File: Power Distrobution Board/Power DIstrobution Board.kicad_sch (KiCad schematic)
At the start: 2 parts, among them J2 Conn_01x10_Pin, J4 Conn_01x04_Pin

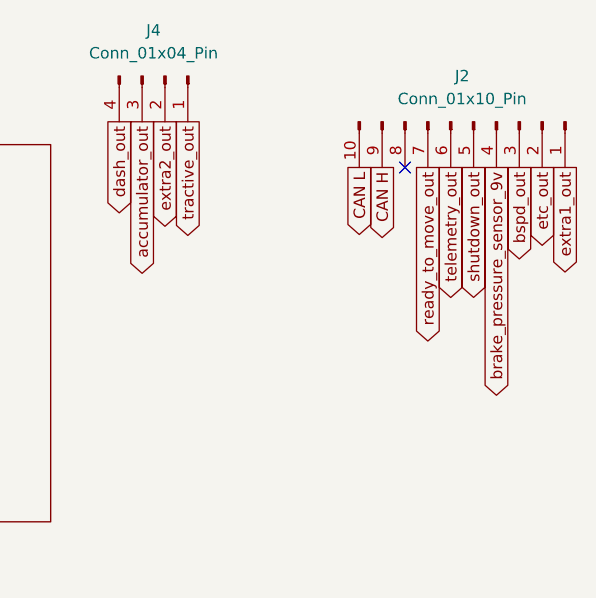
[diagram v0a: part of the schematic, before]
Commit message: version 1.1
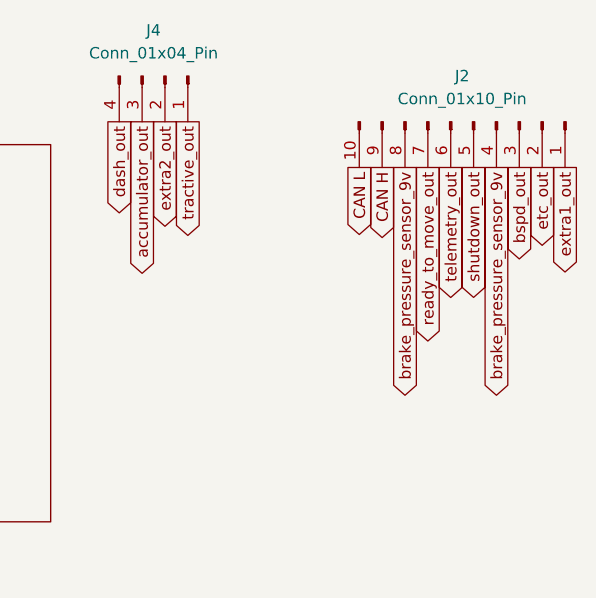
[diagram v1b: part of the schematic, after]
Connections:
- net brake_pressure_sensor_9v: now also J2.8 (Pin_8)
- no-connect marks 1 -> 0
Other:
- company: (none) -> Formula Slug
- title: (none) -> PD BOARD
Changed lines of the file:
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@@
 	(generator_version "8.0")
 	(paper "A4")
-	(no_connect
-		(at 262.89 71.12)
+	(title_block
+		(title "PD BOARD")
+		(date "2024-11-11")
+		(rev "1.1")
+		(company "Formula Slug")
 	)
 	(global_label "CAN H"
@@
 		)
 	)
+	(global_label "brake_pressure_sensor_9v"
+		(shape output)
+		(at 273.05 71.12 270)
+		(fields_autoplaced yes)
+		(effects
+			(font
+				(size 1.27 1.27)
+			)
+			(justify right)
+		)
+		(property "Intersheetrefs" "${INTERSHEET_REFS}"
+			(at 273.05 98.7188 90)
+			(effects
+				(font
+					(size 1.27 1.27)
+				)
+				(justify right)
+				(hide yes)
+			)
+		)
+	)
+	(global_label "brake_pressure_sensor_9v"
+		(shape output)
+		(at 262.89 71.12 270)
+		(fields_autoplaced yes)
+		(effects
+			(font
+				(size 1.27 1.27)
+			)
+			(justify right)
+		)
+		(property "Intersheetrefs" "${INTERSHEET_REFS}"
+			(at 262.89 98.7188 90)
+			(effects
+				(font
+					(size 1.27 1.27)
+				)
+				(justify right)
+				(hide yes)
+			)
+		)
+	)
 	(global_label "dash_out"
 		(shape output)
@@
 			(effects
 				(font
-					(size 1.27 1.27)
-				)
-				(justify right)
-				(hide yes)
-			)
-		)
-	)
-	(global_label "brake_pressure_sensor_9v"
-		(shape output)
-		(at 273.05 71.12 270)
-		(fields_autoplaced yes)
-		(effects
-			(font
-				(size 1.27 1.27)
-			)
-			(justify right)
-		)
-		(property "Intersheetrefs" "${INTERSHEET_REFS}"
-			(at 273.05 98.7188 90)
-			(effects
-				(font

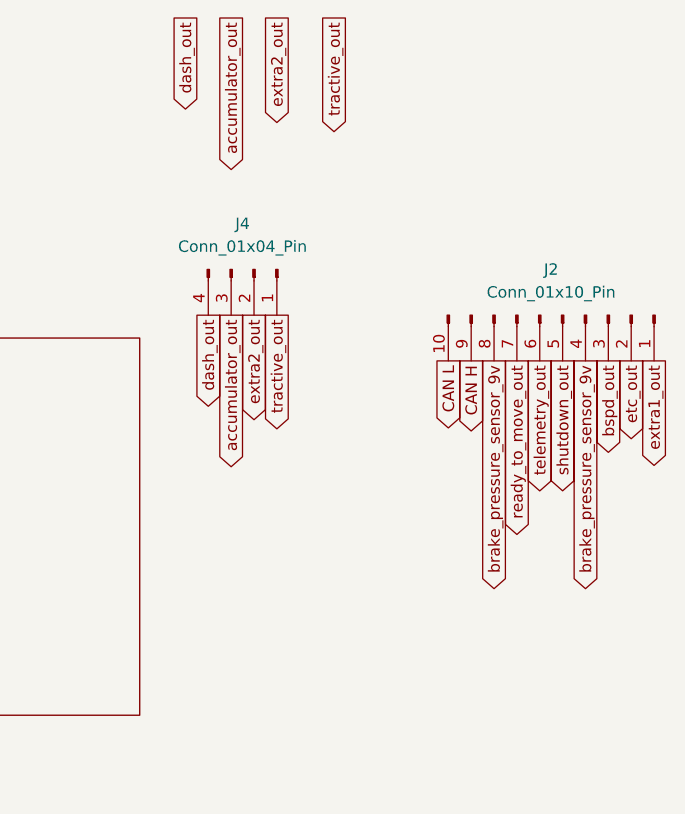
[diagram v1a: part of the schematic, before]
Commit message: even newer changes
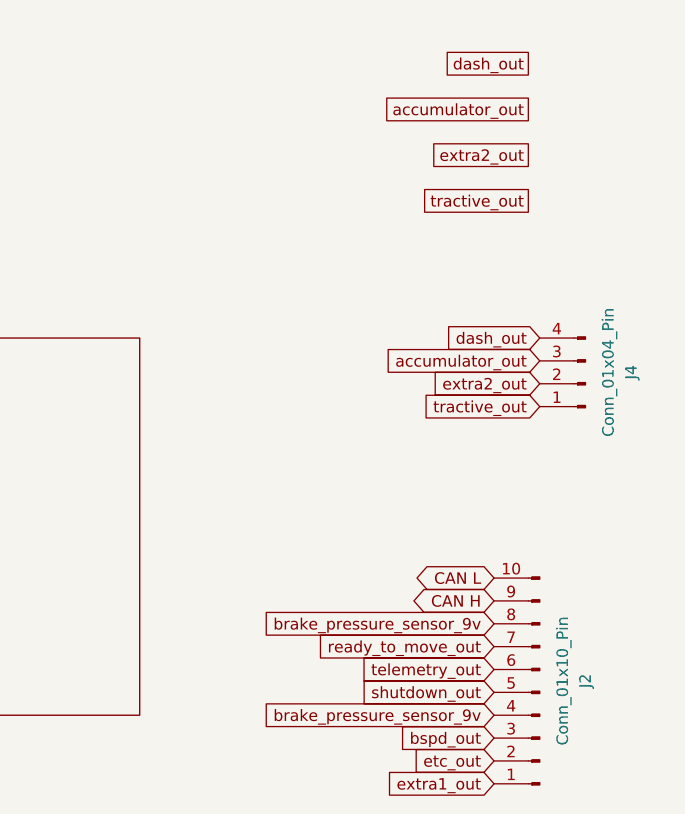
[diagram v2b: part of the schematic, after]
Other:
- moved on the sheet: J2, J4

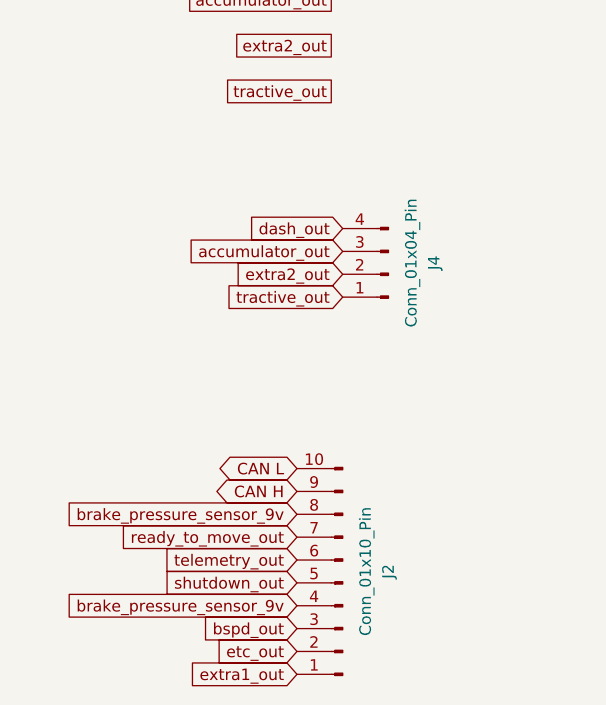
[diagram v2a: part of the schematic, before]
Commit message: commit 1 of v2
pd board v2 work first commit
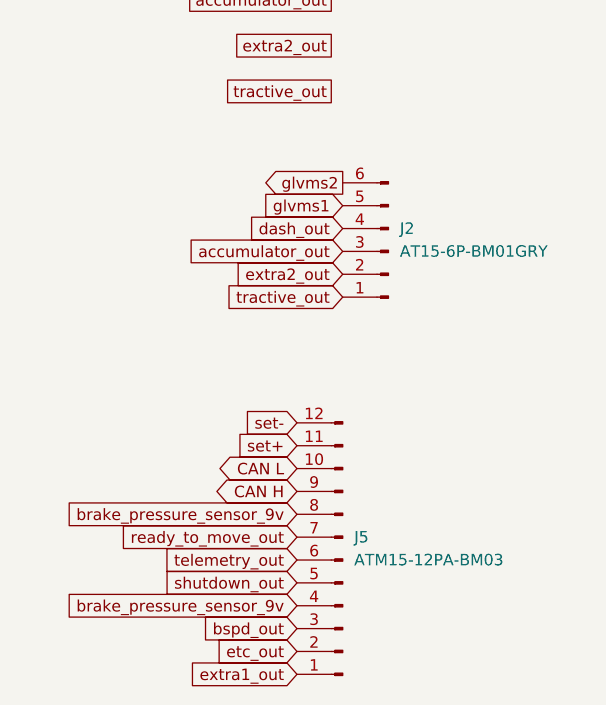
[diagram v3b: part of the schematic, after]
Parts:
- removed J2: Conn_01x10_Pin, Connector_Molex:Molex_Nano-Fit_105314-xx10_2x05_P2.50mm_Horizontal, symbol Connector:Conn_01x10_Pin
- removed J4: Conn_01x04_Pin, Connector_Molex:Molex_Mega-Fit_76825-0004_2x02_P5.70mm_Horizontal, symbol Connector:Conn_01x04_Pin
- added J2: AT15-6P-BM01GRY, FS_3_Global_Footprint_Library:CONN6_DT15-6P_TEC, symbol Connector:Conn_01x06_Pin
- added J5: ATM15-12PA-BM03, FS_3_Global_Footprint_Library:TE_DTM15-12PA, symbol Connector:Conn_01x12_Pin
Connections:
- net CAN H: now also J5.9 (Pin_9)
- net CAN L: now also J5.10 (Pin_10)
- net accumulator_out: now also J2.3 (Pin_3)
- net brake_pressure_sensor_9v: now also J5.4 (Pin_4), J5.8 (Pin_8)
- net bspd_out: now also J5.3 (Pin_3)
- net dash_out: now also J2.4 (Pin_4)
- net etc_out: now also J5.2 (Pin_2)
- net extra1_out: now also J5.1 (Pin_1)
- net extra2_out: now also J2.2 (Pin_2)
- net ready_to_move_out: now also J5.7 (Pin_7)
- net shutdown_out: now also J5.5 (Pin_5)
- net telemetry_out: now also J5.6 (Pin_6)
- net tractive_out: now also J2.1 (Pin_1)
- new net glvms1: J2.5 (Pin_5)
- new net glvms2: J2.6 (Pin_6)
- new net set+: J5.11 (Pin_11)
- new net set-: J5.12 (Pin_12)
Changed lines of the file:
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@@
+		)
+	)
+	(global_label "extra1_out"
+		(shape input)
+		(at 262.89 118.11 180)
+		(fields_autoplaced yes)
+		(effects
+			(font
+				(size 1.27 1.27)
+			)
+			(justify right)
+		)
+		(property "Intersheetrefs" "${INTERSHEET_REFS}"
+			(at 249.9264 118.11 0)
+			(effects
+				(font
+					(size 1.27 1.27)
+				)
+				(justify right)
+				(hide yes)
+			)
 		)
 	)
@@
 		)
 	)
-	(global_label "extra1_out"
-		(shape input)
-		(at 262.89 118.11 180)
-		(fields_autoplaced yes)
-		(effects
-			(font
-				(size 1.27 1.27)
-			)
-			(justify right)
-		)
-		(property "Intersheetrefs" "${INTERSHEET_REFS}"
-			(at 249.9264 118.11 0)
-			(effects
-				(font
-					(size 1.27 1.27)
-				)
-				(justify right)
-				(hide yes)
-			)
-		)
-	)
 	(global_label "etc_out"
 		(shape input)
@@
 		(property "Intersheetrefs" "${INTERSHEET_REFS}"
 			(at 253.0106 115.57 0)
+			(effects
+				(font
+					(size 1.27 1.27)
+				)
+				(justify right)
+				(hide yes)
+			)
+		)
+	)
+	(global_label "glvms1"
+		(shape input)
+		(at 267.97 66.04 180)
+		(fields_autoplaced yes)
+		(effects
+			(font
+				(size 1.27 1.27)
+			)
+			(justify right)
+		)
+		(property "Intersheetrefs" "${INTERSHEET_REFS}"
+			(at 258.2721 66.04 0)
 			(effects
 				(font
@@
 		)
 	)
+	(global_label "set+"
+		(shape input)
+		(at 262.89 92.71 180)
+		(fields_autoplaced yes)
+		(effects
+			(font
+				(size 1.27 1.27)
+			)
+			(justify right)
+		)
+		(property "Intersheetrefs" "${INTERSHEET_REFS}"
+			(at 255.49 92.71 0)
+			(effects
+				(font
+					(size 1.27 1.27)
+				)
+				(justify right)
+				(hide yes)
+			)
+		)
+	)
 	(global_label "ready_to_move_out"
 		(shape input)
@@
 		)
 	)
+	(global_label "glvms2"
+		(shape output)
+		(at 267.97 63.5 180)
+		(fields_autoplaced yes)
+		(effects
+			(font
+				(size 1.27 1.27)
+			)
+			(justify right)
+		)
+		(property "Intersheetrefs" "${INTERSHEET_REFS}"
+			(at 258.2721 63.5 0)
+			(effects
+				(font
+					(size 1.27 1.27)
+				)
+				(justify right)
+				(hide yes)
+			)
+		)
+	)
 	(global_label "shutdown_out"
 		(shape input)
@@
 		(property "Intersheetrefs" "${INTERSHEET_REFS}"
 			(at 253.8573 76.2 0)
+			(effects
+				(font
+					(size 1.27 1.27)
+				)
+				(justify right)
+				(hide yes)
+			)
+		)
+	)
+	(global_label "set-"
+		(shape input)
+		(at 262.89 90.17 180)
+		(fields_autoplaced yes)
+		(effects
+			(font
+				(size 1.27 1.27)
+			)
+			(justify right)
+		)
+		(property "Intersheetrefs" "${INTERSHEET_REFS}"
+			(at 255.49 90.17 0)
 			(effects
 				(font
@@
 	)
 	(symbol
-		(lib_id "Connector:Conn_01x10_Pin")
-		(at 267.97 107.95 180)
+		(lib_id "Connector:Conn_01x12_Pin")
+		(at 267.97 105.41 180)
 		(unit 1)
 		(exclude_from_sim no)
@@
 		(dnp no)
 		(fields_autoplaced yes)
+		(property "Reference" "J5"
+			(at 269.24 102.8699 0)
+			(effects
+				(font
+					(size 1.27 1.27)
+				)
+				(justify right)
+			)
+		)
+		(property "Value" "ATM15-12PA-BM03"
+			(at 269.24 105.4099 0)
+			(effects
+				(font
+					(size 1.27 1.27)
+				)
+				(justify right)
+			)
+		)
+		(property "Footprint" "FS_3_Global_Footprint_Library:TE_DTM15-12PA"
+			(at 267.97 105.41 0)
+			(effects
+				(font
+					(size 1.27 1.27)
+				)
+				(hide yes)
+			)
+		)
+		(property "Datasheet" "~"
+			(at 267.97 105.41 0)
+			(effects
+				(font
+					(size 1.27 1.27)
+				)
+				(hide yes)
+			)
+		)
+		(property "Description" "Generic connector, single row, 01x12, script generated"
+			(at 267.97 105.41 0)
+			(effects
+				(font
+					(size 1.27 1.27)
+				)
+				(hide yes)
+			)
+		)
+		(pin "7"
+		)
+		(pin "11"
+		)
+		(pin "4"
+		)
+		(pin "6"
+		)
+		(pin "1"
+		)
+		(pin "3"
+		)
+		(pin "2"
+		)
+		(pin "12"
+		)
+		(pin "5"
+		)
+		(pin "10"
+		)
+		(pin "9"
+		)
+		(pin "8"
+		)
+		(instances
+			(project ""
+				(path "/cd827802-ab32-49ad-ad84-bccf81c569e7"
+					(reference "J5")
+					(unit 1)
+				)
+			)
+		)
+	)
+	(symbol
+		(lib_id "Connector:Conn_01x06_Pin")
+		(at 273.05 71.12 180)
+		(unit 1)
+		(exclude_from_sim no)
+		(in_bom yes)
+		(on_board yes)
+		(dnp no)
+		(fields_autoplaced yes)
 		(property "Reference" "J2"
-			(at 273.05 106.68 90)
-			(effects
-				(font
-					(size 1.27 1.27)
-				)
-			)
-		)
-		(property "Value" "Conn_01x10_Pin"
-			(at 270.51 106.68 90)
-			(effects
-				(font
-					(size 1.27 1.27)
-				)
-			)
-		)
-		(property "Footprint" "Connector_Molex:Molex_Nano-Fit_105314-xx10_2x05_P2.50mm_Horizontal"
-			(at 267.97 107.95 0)
-			(effects
-				(font
-					(size 1.27 1.27)
-				)
-				(hide yes)
-			)
-		)
-		(property "Datasheet" "https://www.molex.com/content/dam/molex/molex-dot-com/en_us/pdf/datasheets/987651-1223.pdf"
-			(at 267.97 107.95 0)
-			(effects
-				(font
-					(size 1.27 1.27)
-				)
-				(hide yes)
-			)
-		)
-		(property "Description" "Generic connector, single row, 01x10, script generated"
-			(at 267.97 107.95 0)
-			(effects
-				(font
-					(size 1.27 1.27)
-				)
-				(hide yes)
-			)
-		)
-		(pin "8"
+			(at 274.32 68.5799 0)
+			(effects
+				(font
+					(size 1.27 1.27)
+				)
+				(justify right)
+			)
+		)
+		(property "Value" "AT15-6P-BM01GRY"
+			(at 274.32 71.1199 0)
+			(effects
+				(font
+					(size 1.27 1.27)
+				)
+				(justify right)
+			)
+		)
+		(property "Footprint" "FS_3_Global_Footprint_Library:CONN6_DT15-6P_TEC"
+			(at 273.05 71.12 0)
+			(effects
+				(font
+					(size 1.27 1.27)
+				)
+				(hide yes)
+			)
+		)
+		(property "Datasheet" "~"
+			(at 273.05 71.12 0)
+			(effects
+				(font
+					(size 1.27 1.27)
+				)
+				(hide yes)
+			)
+		)
+		(property "Description" "Generic connector, single row, 01x06, script generated"
+			(at 273.05 71.12 0)
+			(effects
+				(font
+					(size 1.27 1.27)
+				)
+				(hide yes)
+			)
+		)
+		(pin "1"
 		)
 		(pin "2"
 		)
+		(pin "3"
+		)
 		(pin "4"
 		)
-		(pin "3"
-		)
-		(pin "1"
-		)
-		(pin "7"
-		)
-		(pin "9"
+		(pin "5"
 		)
 		(pin "6"
-		)
-		(pin "5"
-		)
-		(pin "10"
 		)
 		(instances
@@
 					(unit 1)
 				)
-			)
-		)
-	)
-	(symbol
-		(lib_id "Connector:Conn_01x04_Pin")
-		(at 273.05 73.66 180)
-		(unit 1)
-		(exclude_from_sim no)
-		(in_bom yes)
-		(on_board yes)
-		(dnp no)
-		(fields_autoplaced yes)
-		(property "Reference" "J4"
-			(at 278.13 72.39 90)
-			(effects
-				(font
-					(size 1.27 1.27)
-				)
-			)
-		)
-		(property "Value" "Conn_01x04_Pin"
-			(at 275.59 72.39 90)
-			(effects
-				(font
-					(size 1.27 1.27)
-				)
-			)
-		)
-		(property "Footprint" "Connector_Molex:Molex_Mega-Fit_76825-0004_2x02_P5.70mm_Horizontal"
-			(at 273.05 73.66 0)
-			(effects
-				(font
-					(size 1.27 1.27)
-				)
-				(hide yes)
-			)
-		)
-		(property "Datasheet" "https://tools.molex.com/pdm_docs/ps/PS-76823-100.pdf"
-			(at 273.05 73.66 0)
-			(effects
-				(font
-					(size 1.27 1.27)
-				)
-				(hide yes)
-			)
-		)
-		(property "Description" "Generic connector, single row, 01x04, script generated"
-			(at 273.05 73.66 0)
-			(effects
-				(font
-					(size 1.27 1.27)
-				)
-				(hide yes)
-			)
-		)
-		(pin "4"
-		)
-		(pin "1"
-		)
-		(pin "3"
-		)
-		(pin "2"
-		)
-		(instances
-			(project ""
-				(path "/cd827802-ab32-49ad-ad84-bccf81c569e7"
-					(reference "J4")
-					(unit 1)
-				)

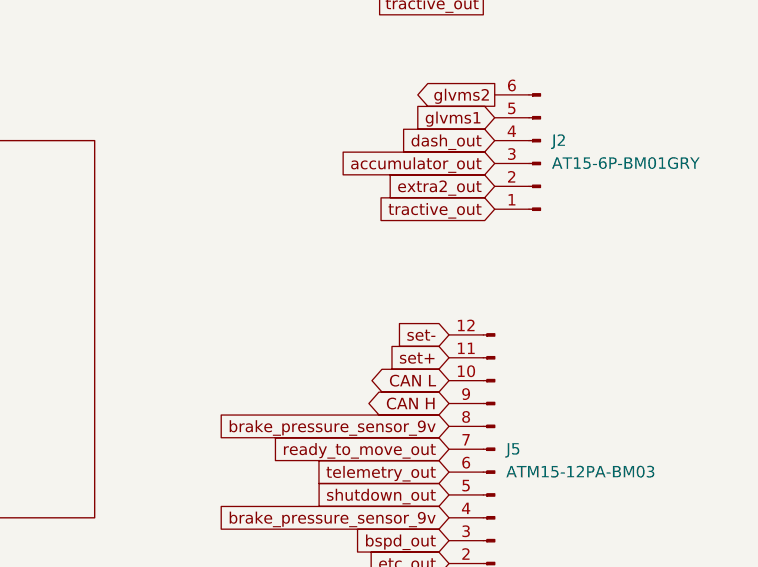
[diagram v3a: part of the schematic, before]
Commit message: v2 3/29
almost done need to add mounting holes text, clean up screen printing, and get linear regs re speced
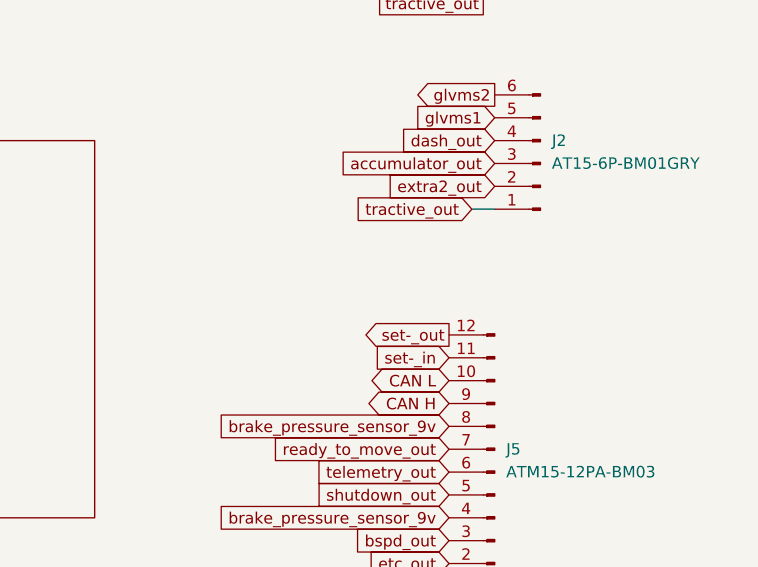
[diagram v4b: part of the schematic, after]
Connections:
- net set+ renamed set-_in
- net set- renamed set-_out
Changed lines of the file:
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@@
 		(company "Formula Slug")
+	)
+	(wire
+		(pts
+			(xy 265.43 76.2) (xy 267.97 76.2)
+		)
+		(stroke
+			(width 0)
+			(type default)
+		)
 	)
 	(global_label "CAN H"
@@
 		)
 	)
-	(global_label "set+"
+	(global_label "set-_in"
 		(shape input)
 		(at 262.89 92.71 180)
@@
 		)
 		(property "Intersheetrefs" "${INTERSHEET_REFS}"
-			(at 255.49 92.71 0)
+			(at 252.7686 92.71 0)
 			(effects
 				(font
@@
 	(global_label "tractive_out"
 		(shape input)
-		(at 267.97 76.2 180)
-		(fields_autoplaced yes)
-		(effects
-			(font
-				(size 1.27 1.27)
-			)
-			(justify right)
-		)
-		(property "Intersheetrefs" "${INTERSHEET_REFS}"
-			(at 253.8573 76.2 0)
-			(effects
-				(font
-					(size 1.27 1.27)
-				)
-				(justify right)
-				(hide yes)
-			)
-		)
-	)
-	(global_label "set-"
-		(shape input)
+		(at 265.43 76.2 180)
+		(fields_autoplaced yes)
+		(effects
+			(font
+				(size 1.27 1.27)
+			)
+			(justify right)
+		)
+		(property "Intersheetrefs" "${INTERSHEET_REFS}"
+			(at 251.3173 76.2 0)
+			(effects
+				(font
+					(size 1.27 1.27)
+				)
+				(justify right)
+				(hide yes)
+			)
+		)
+	)
+	(global_label "set-_out"
+		(shape output)
 		(at 262.89 90.17 180)
 		(fields_autoplaced yes)
@@
 		)
 		(property "Intersheetrefs" "${INTERSHEET_REFS}"
-			(at 255.49 90.17 0)
+			(at 251.4987 90.17 0)
 			(effects
 				(font
@@
 			(effects
 				(font
+					(size 1.27 1.27)
+					(italic yes)
+				)
+				(justify left)
+			)
+		)
+	)
+	(netclass_flag ""
+		(length 2.54)
+		(shape round)
+		(at 266.7 76.2 180)
+		(fields_autoplaced yes)
+		(effects
+			(font
+				(size 1.27 1.27)
+			)
+			(justify right bottom)
+		)
+		(property "Netclass" "10A"
+			(at 267.3985 78.74 0)
+			(effects
+				(font

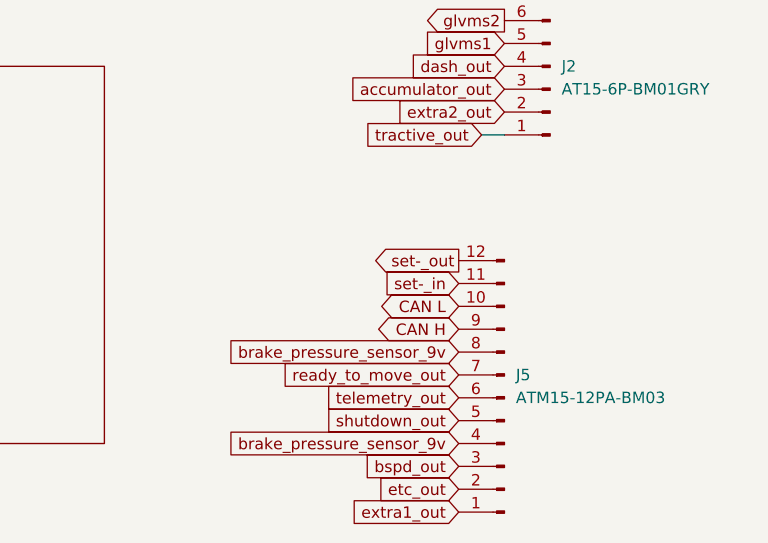
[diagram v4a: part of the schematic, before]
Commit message: another push idk
idk what changed i just saved some stuff
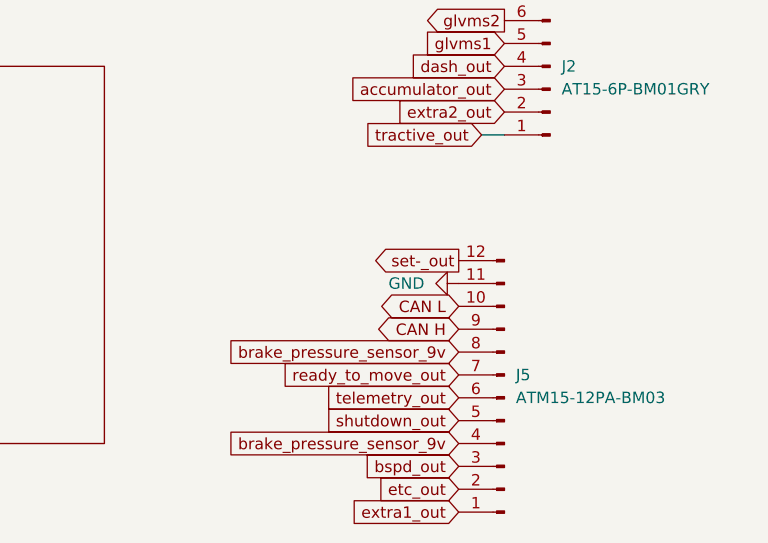
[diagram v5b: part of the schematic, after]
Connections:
- net set-_in renamed GND
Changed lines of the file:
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@@
-		)
-	)
-	(global_label "set-_in"
-		(shape input)
-		(at 262.89 92.71 180)
-		(fields_autoplaced yes)
-		(effects
-			(font
-				(size 1.27 1.27)
-			)
-			(justify right)
-		)
-		(property "Intersheetrefs" "${INTERSHEET_REFS}"
-			(at 252.7686 92.71 0)
-			(effects
-				(font
-					(size 1.27 1.27)
-				)
-				(justify right)
-				(hide yes)
-			)
 		)
 	)
@@
 					(unit 1)
 				)
+			)
+		)
+	)
+	(symbol
+		(lib_id "power:GND")
+		(at 262.89 92.71 270)
+		(unit 1)
+		(exclude_from_sim no)
+		(in_bom yes)
+		(on_board yes)
+		(dnp no)
+		(fields_autoplaced yes)
+		(property "Reference" "#PWR076"
+			(at 256.54 92.71 0)
+			(effects
+				(font
+					(size 1.27 1.27)
+				)
+				(hide yes)
+			)
+		)
+		(property "Value" "GND"
+			(at 259.08 92.7099 90)
+			(effects
+				(font
+					(size 1.27 1.27)
+				)
+				(justify right)
+			)
+		)
+		(property "Footprint" ""
+			(at 262.89 92.71 0)
+			(effects
+				(font
+					(size 1.27 1.27)
+				)
+				(hide yes)
+			)
+		)
+		(property "Datasheet" ""
+			(at 262.89 92.71 0)
+			(effects
+				(font
+					(size 1.27 1.27)
+				)
+				(hide yes)
+			)
+		)
+		(property "Description" "Power symbol creates a global label with name \"GND\" , ground"
+			(at 262.89 92.71 0)
+			(effects
+				(font
+					(size 1.27 1.27)
+				)
+				(hide yes)
+			)
+		)
+		(pin "1"
+		)
+		(instances
+			(project ""
+				(path "/cd827802-ab32-49ad-ad84-bccf81c569e7"
+					(reference "#PWR076")
+					(unit 1)
+				)
